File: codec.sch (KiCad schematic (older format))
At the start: 11 parts, among them U1 WM8778

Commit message: ksch: add stuff that isn't on soldered prototype yet
this hopefully completes the rev. A schematics
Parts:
- removed U1: WM8778, symbol WM8778
- removed U?: WM8778-units, symbol WM8778-units
- added C2: 0.1u, Capacitors_SMD:C_0805_HandSoldering, symbol C_Small
- added C3: 0.01u, Capacitors_SMD:C_0805_HandSoldering, symbol C_Small
- added C4: 1u, Capacitors_SMD:C_0805_HandSoldering, symbol C_Small
- added C5: 100p, Capacitors_SMD:C_0805_HandSoldering, symbol C_Small
- added C6, C7: 4.7nF, Capacitors_SMD:C_0805_HandSoldering, symbol C_Small
- added C8, C9: 10u, Capacitors_SMD:C_0805_HandSoldering, symbol C_Small
- added J1: electret mic, Socket_Strips:Socket_Strip_Straight_1x02_Pitch2.54mm, symbol CONN_01X02
- added J2: line in, Socket_Strips:Socket_Strip_Straight_1x03_Pitch2.54mm, symbol JACK_2P
- added J3: line/~mic, Connectors:GS2, symbol GS2
- added J5: JACK_3P, Socket_Strips:Socket_Strip_Straight_1x03_Pitch2.54mm, symbol JACK_3P
- added R10: 10k, Resistors_THT:R_Axial_DIN0207_L6.3mm_D2.5mm_P7.62mm_Horizontal, symbol R_Small
- added R11: 100k, Resistors_THT:R_Axial_DIN0207_L6.3mm_D2.5mm_P7.62mm_Horizontal, symbol R_Small
- added R12, R13: 680, Resistors_THT:R_Axial_DIN0207_L6.3mm_D2.5mm_P7.62mm_Horizontal, symbol R_Small
- added R5: 1k, Resistors_THT:R_Axial_DIN0207_L6.3mm_D2.5mm_P7.62mm_Horizontal, symbol R_Small
- added R6, R7: 2k, Resistors_THT:R_Axial_DIN0207_L6.3mm_D2.5mm_P7.62mm_Horizontal, symbol R_Small
- added R8, R9: 1M, Resistors_THT:R_Axial_DIN0207_L6.3mm_D2.5mm_P7.62mm_Horizontal, symbol R_Small
- added U2: MAX4466, TO_SOT_Packages_SMD:SOT-353_SC-70-5_Handsoldering, symbol MAX4466
- C401, C402: renamed from C?; footprint (none) -> Capacitors_THT:CP_Radial_D5.0mm_P2.00mm
- C403, C404: renamed from C?; footprint (none) -> Capacitors_THT:CP_Radial_D4.0mm_P2.00mm
- R401, R402, R403, R404: renamed from R?; footprint (none) -> Resistors_THT:R_Axial_DIN0207_L6.3mm_D2.5mm_P7.62mm_Horizontal
- U201: renamed from U?; footprint (none) -> footprints:SSOP-28_5.3x10.2mm_Pitch0.65mm_HandSolder
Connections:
- net labels removed: 3.3V, 5V, DGND
- wire segments 10 -> 46
- no-connect marks 28 -> 0
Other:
- note removed: "HIGH: I2S Mode\nLOW: 2pin Mode\nFLOAT: Hardware Mode"

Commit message: ksch: reannotate schematics to have a single style of part-naming
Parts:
- renumbered C2 to C34, C3 to C35, C4 to C36, C5 to C37, C6 to C38, C7 to C39, C8 to C40, C9 to C41, C401 to C42, C402 to C43, C403 to C44, C404 to C45, J1 to J5, J2 to J6, J3 to J7, J5 to J8, R7 to R10, R8 to R11, R9 to R12, R10 to R13, R11 to R14, R12 to R15, R13 to R16, R401 to R17, R402 to R18, R403 to R19, R404 to R20, R5 to R8, R6 to R9, U201 to U1, U2 to U7

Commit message: ksch: fix footprintproblem, change some labels
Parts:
- J8: value JACK_3P -> stereo_out
- U7: footprint TO_SOT_Packages_SMD:SOT-353_SC-70-5_Handsoldering -> footprints:SOT-353_SC-70-5_Handsoldering
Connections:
- net labels added: 5V, voutl, voutr
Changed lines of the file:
@@
 LIBS:ftdi
 LIBS:gennum
-LIBS:graphic
 LIBS:hc11
 LIBS:intel
@@
 LIBS:leds
 LIBS:linear
-LIBS:logo
 LIBS:maxim
 LIBS:mechanical
@@
 F 0 "U7" H 3550 2850 50  0000 L CNN
 F 1 "MAX4466" H 3550 2550 50  0000 L CNN
-F 2 "TO_SOT_Packages_SMD:SOT-353_SC-70-5_Handsoldering" H 3550 2550 50  0001 L CNN
+F 2 "footprints:SOT-353_SC-70-5_Handsoldering" H 3550 2550 50  0001 L CNN
 F 3 "" H 3700 2850 50  0001 C CNN
 	1    3550 2700
@@
 P 10050 3450
 F 0 "J8" H 9572 3433 50  0000 R CNN
-F 1 "JACK_3P" H 9572 3524 50  0000 R CNN
+F 1 "stereo_out" H 9572 3524 50  0000 R CNN
 F 2 "Socket_Strips:Socket_Strip_Straight_1x03_Pitch2.54mm" H 10050 3450 50  0001 C CNN
 F 3 "" H 10050 3450 50  0001 C CNN
@@
 Wire Wire Line
 	8650 3450 8650 3900
+Text Label 8850 3450 0    60   ~ 0
+voutl
+Text Label 8850 3100 0    60   ~ 0
+voutr
+Text GLabel 3450 2100 2    60   Input ~ 0
+5V
 $EndSCHEMATC

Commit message: k: fix pcb
power connector trouble
wrong footprint for caps
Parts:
- C44, C45: footprint Capacitors_THT:CP_Radial_D4.0mm_P2.00mm -> Capacitors_SMD:C_0805_HandSoldering
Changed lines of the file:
@@
 F 0 "C45" H 7960 4070 50  0000 L CNN
 F 1 "4.7nF" H 7960 3920 50  0000 L CNN
-F 2 "Capacitors_THT:CP_Radial_D4.0mm_P2.00mm" H 7950 4000 50  0001 C CNN
+F 2 "Capacitors_SMD:C_0805_HandSoldering" H 7950 4000 50  0001 C CNN
 F 3 "" H 7950 4000 50  0001 C CNN
 	1    7950 4000
@@
 F 0 "C44" H 7960 3270 50  0000 L CNN
 F 1 "4.7nF" H 7960 3120 50  0000 L CNN
-F 2 "Capacitors_THT:CP_Radial_D4.0mm_P2.00mm" H 7950 3200 50  0001 C CNN
+F 2 "Capacitors_SMD:C_0805_HandSoldering" H 7950 3200 50  0001 C CNN
 F 3 "" H 7950 3200 50  0001 C CNN
 	1    7950 3200

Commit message: ksch: change component values to include the unit except for resistors add more info to some devices
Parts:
- C34: value 0.1u -> 100nF
- C35: value 0.01u -> 10nF C0G/NP0
- C36: value 1u -> 1uF
- C37: value 100p -> 100pF
- C38, C39, C44, C45: value 4.7nF -> 4.7nF C0G/NP0
- C40, C41: value 10u -> 10uF C0G/NP0
- C42, C43: value 10uF -> 10uF C0G/NP0
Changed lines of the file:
@@
 Sheet 4 4
 Title "OpenLoop"
-Date "2017-09-25"
+Date "2017-10-02"
 Rev "A"
 Comp ""
@@
 P 7450 3900
 F 0 "C43" H 7475 4000 50  0000 L CNN
-F 1 "10uF" H 7475 3800 50  0000 L CNN
+F 1 "10uF C0G/NP0" H 7475 3800 50  0000 L CNN
 F 2 "Capacitors_THT:CP_Radial_D5.0mm_P2.00mm" H 7488 3750 50  0001 C CNN
 F 3 "" H 7450 3900 50  0001 C CNN
@@
 P 7950 4000
 F 0 "C45" H 7960 4070 50  0000 L CNN
-F 1 "4.7nF" H 7960 3920 50  0000 L CNN
+F 1 "4.7nF C0G/NP0" H 7960 3920 50  0000 L CNN
 F 2 "Capacitors_SMD:C_0805_HandSoldering" H 7950 4000 50  0001 C CNN
 F 3 "" H 7950 4000 50  0001 C CNN
@@
 P 7450 3100
 F 0 "C42" H 7475 3200 50  0000 L CNN
-F 1 "10uF" H 7475 3000 50  0000 L CNN
+F 1 "10uF C0G/NP0" H 7475 3000 50  0000 L CNN
 F 2 "Capacitors_THT:CP_Radial_D5.0mm_P2.00mm" H 7488 2950 50  0001 C CNN
 F 3 "" H 7450 3100 50  0001 C CNN
@@
 P 7950 3200
 F 0 "C44" H 7960 3270 50  0000 L CNN
-F 1 "4.7nF" H 7960 3120 50  0000 L CNN
+F 1 "4.7nF C0G/NP0" H 7960 3120 50  0000 L CNN
 F 2 "Capacitors_SMD:C_0805_HandSoldering" H 7950 3200 50  0001 C CNN
 F 3 "" H 7950 3200 50  0001 C CNN
@@
 P 3000 3100
 F 0 "C36" H 3010 3170 50  0000 L CNN
-F 1 "1u" H 3010 3020 50  0000 L CNN
+F 1 "1uF" H 3010 3020 50  0000 L CNN
 F 2 "Capacitors_SMD:C_0805_HandSoldering" H 3000 3100 50  0001 C CNN
 F 3 "" H 3000 3100 50  0001 C CNN
@@
 P 3450 3350
 F 0 "C37" H 3460 3420 50  0000 L CNN
-F 1 "100p" H 3460 3270 50  0000 L CNN
+F 1 "100pF" H 3460 3270 50  0000 L CNN
 F 2 "Capacitors_SMD:C_0805_HandSoldering" H 3450 3350 50  0001 C CNN
 F 3 "" H 3450 3350 50  0001 C CNN
@@
 P 2300 2600
 F 0 "C35" H 2310 2670 50  0000 L CNN
-F 1 "0.01u" H 2310 2520 50  0000 L CNN
+F 1 "10nF C0G/NP0" H 2310 2520 50  0000 L CNN
 F 2 "Capacitors_SMD:C_0805_HandSoldering" H 2300 2600 50  0001 C CNN
 F 3 "" H 2300 2600 50  0001 C CNN
@@
 P 1900 2750
 F 0 "C34" H 1910 2820 50  0000 L CNN
-F 1 "0.1u" H 1910 2670 50  0000 L CNN
+F 1 "100nF" H 1910 2670 50  0000 L CNN
 F 2 "Capacitors_SMD:C_0805_HandSoldering" H 1900 2750 50  0001 C CNN
 F 3 "" H 1900 2750 50  0001 C CNN
@@
 P 4450 3300
 F 0 "C38" H 4460 3370 50  0000 L CNN
-F 1 "4.7nF" H 4460 3220 50  0000 L CNN
+F 1 "4.7nF C0G/NP0" H 4460 3220 50  0000 L CNN
 F 2 "Capacitors_SMD:C_0805_HandSoldering" H 4450 3300 50  0001 C CNN
 F 3 "" H 4450 3300 50  0001 C CNN
@@
 P 4950 3350
 F 0 "C40" H 4960 3420 50  0000 L CNN
-F 1 "10u" H 4960 3270 50  0000 L CNN
+F 1 "10uF C0G/NP0" H 4960 3270 50  0000 L CNN
 F 2 "Capacitors_SMD:C_0805_HandSoldering" H 4950 3350 50  0001 C CNN
 F 3 "" H 4950 3350 50  0001 C CNN
@@
 P 4450 3750
 F 0 "C39" H 4460 3820 50  0000 L CNN
-F 1 "4.7nF" H 4460 3670 50  0000 L CNN
+F 1 "4.7nF C0G/NP0" H 4460 3670 50  0000 L CNN
 F 2 "Capacitors_SMD:C_0805_HandSoldering" H 4450 3750 50  0001 C CNN
 F 3 "" H 4450 3750 50  0001 C CNN
@@
 P 4950 3650
 F 0 "C41" H 4960 3720 50  0000 L CNN
-F 1 "10u" H 4960 3570 50  0000 L CNN
+F 1 "10uF C0G/NP0" H 4960 3570 50  0000 L CNN
 F 2 "Capacitors_SMD:C_0805_HandSoldering" H 4950 3650 50  0001 C CNN
 F 3 "" H 4950 3650 50  0001 C CNN

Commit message: migrate to kicad v5
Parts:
- C34, C35, C36, C37, C38, C39, C40, C41, C44, C45: symbol C_Small -> Device:C_Small
- C42, C43: symbol CP -> Device:CP
- J5: symbol CONN_01X02 -> Connector:Conn_01x02_Male
- J6: symbol JACK_2P -> Connector:AudioJack2_Ground_Switch
- J7: symbol GS2 -> Connector:TestPoint_2Pole
- J8: symbol JACK_3P -> openloop:JACK_3P
- R10, R11, R12, R13, R14, R15, R16, R17, R18, R19, R20, R8, R9: symbol R_Small -> Device:R_Small
- U1: symbol WM8778-units -> openloop:WM8778-units
- U7: symbol MAX4466 -> openloop:MAX4466
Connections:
- wire segments 46 -> 66

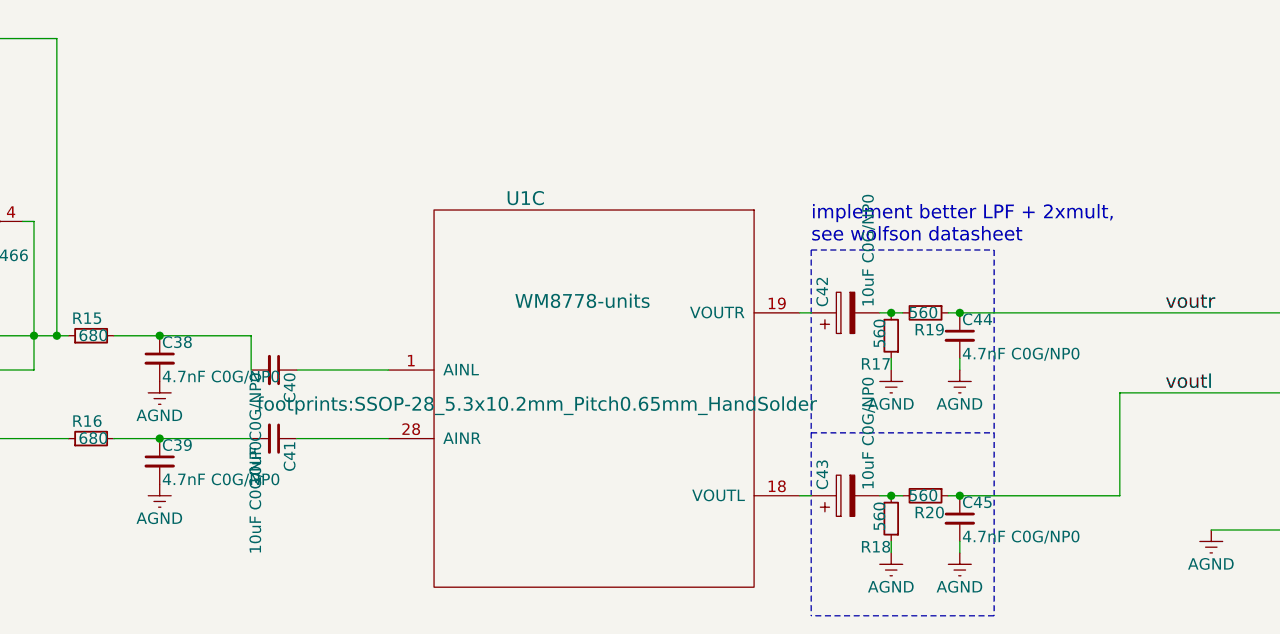
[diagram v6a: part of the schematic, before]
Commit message: ready for print
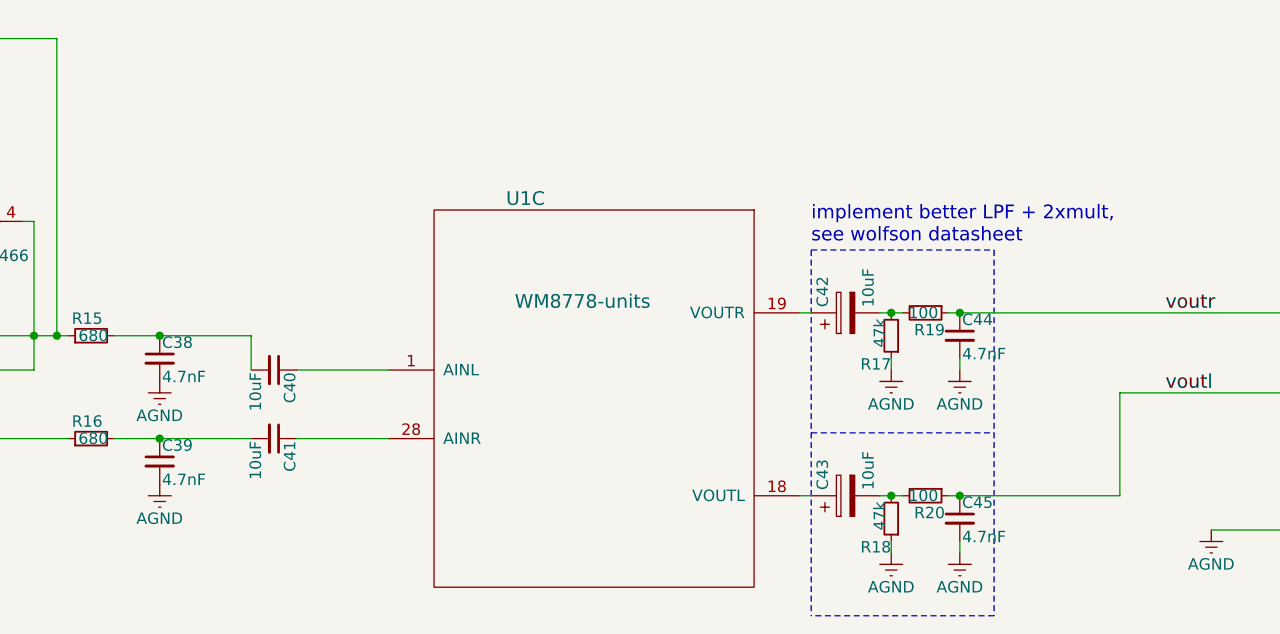
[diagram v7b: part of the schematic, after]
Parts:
- C38, C39, C44, C45: value 4.7nF C0G/NP0 -> 4.7nF
- C40, C41, C42, C43: value 10uF C0G/NP0 -> 10uF
- R17, R18: value 560 -> 47k
- R19, R20: value 560 -> 100
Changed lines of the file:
@@
 Sheet 4 4
 Title "OpenLoop"
-Date "2017-10-02"
+Date "2018-06-20"
 Rev "A"
 Comp ""
@@
 F 0 "U1" H 6050 4400 60  0000 C CNN
 F 1 "WM8778-units" H 6300 3950 60  0000 C CNN
-F 2 "footprints:SSOP-28_5.3x10.2mm_Pitch0.65mm_HandSolder" H 6100 3500 60  0000 C CNN
+F 2 "footprints:SSOP-28_5.3x10.2mm_Pitch0.65mm_HandSolder" H 6100 3500 60  0001 C CNN
 F 3 "" H 6100 3500 60  0000 C CNN
 	3    6350 3500
@@
 P 7800 3900
 F 0 "R20" V 7875 3850 50  0000 L CNN
-F 1 "560" V 7800 3825 50  0000 L CNN
+F 1 "100" V 7800 3825 50  0000 L CNN
 F 2 "Resistors_THT:R_Axial_DIN0207_L6.3mm_D2.5mm_P7.62mm_Horizontal" H 7800 3900 50  0001 C CNN
 F 3 "" H 7800 3900 50  0001 C CNN
@@
 P 7450 3900
 F 0 "C43" H 7475 4000 50  0000 L CNN
-F 1 "10uF C0G/NP0" H 7475 3800 50  0000 L CNN
+F 1 "10uF" H 7475 3800 50  0000 L CNN
 F 2 "Capacitors_THT:CP_Radial_D5.0mm_P2.00mm" H 7488 3750 50  0001 C CNN
 F 3 "" H 7450 3900 50  0001 C CNN
@@
 P 7950 4000
 F 0 "C45" H 7960 4070 50  0000 L CNN
-F 1 "4.7nF C0G/NP0" H 7960 3920 50  0000 L CNN
+F 1 "4.7nF" H 7960 3920 50  0000 L CNN
 F 2 "Capacitors_SMD:C_0805_HandSoldering" H 7950 4000 50  0001 C CNN
 F 3 "" H 7950 4000 50  0001 C CNN
@@
 P 7650 4000
 F 0 "R18" H 7650 4125 50  0000 L CNN
-F 1 "560" V 7700 3925 50  0000 L CNN
+F 1 "47k" V 7700 3925 50  0000 L CNN
 F 2 "Resistors_THT:R_Axial_DIN0207_L6.3mm_D2.5mm_P7.62mm_Horizontal" H 7650 4000 50  0001 C CNN
 F 3 "" H 7650 4000 50  0001 C CNN
@@
 P 7800 3100
 F 0 "R19" V 7875 3050 50  0000 L CNN
-F 1 "560" V 7800 3025 50  0000 L CNN
+F 1 "100" V 7800 3025 50  0000 L CNN
 F 2 "Resistors_THT:R_Axial_DIN0207_L6.3mm_D2.5mm_P7.62mm_Horizontal" H 7800 3100 50  0001 C CNN
 F 3 "" H 7800 3100 50  0001 C CNN
@@
 P 7450 3100
 F 0 "C42" H 7475 3200 50  0000 L CNN
-F 1 "10uF C0G/NP0" H 7475 3000 50  0000 L CNN
+F 1 "10uF" H 7475 3000 50  0000 L CNN
 F 2 "Capacitors_THT:CP_Radial_D5.0mm_P2.00mm" H 7488 2950 50  0001 C CNN
 F 3 "" H 7450 3100 50  0001 C CNN
@@
 P 7950 3200
 F 0 "C44" H 7960 3270 50  0000 L CNN
-F 1 "4.7nF C0G/NP0" H 7960 3120 50  0000 L CNN
+F 1 "4.7nF" H 7960 3120 50  0000 L CNN
 F 2 "Capacitors_SMD:C_0805_HandSoldering" H 7950 3200 50  0001 C CNN
 F 3 "" H 7950 3200 50  0001 C CNN
@@
 P 7650 3200
 F 0 "R17" H 7650 3325 50  0000 L CNN
-F 1 "560" V 7700 3125 50  0000 L CNN
+F 1 "47k" V 7700 3125 50  0000 L CNN
 F 2 "Resistors_THT:R_Axial_DIN0207_L6.3mm_D2.5mm_P7.62mm_Horizontal" H 7650 3200 50  0001 C CNN
 F 3 "" H 7650 3200 50  0001 C CNN
@@
 P 4450 3300
 F 0 "C38" H 4460 3370 50  0000 L CNN
-F 1 "4.7nF C0G/NP0" H 4460 3220 50  0000 L CNN
+F 1 "4.7nF" H 4460 3220 50  0000 L CNN
 F 2 "Capacitors_SMD:C_0805_HandSoldering" H 4450 3300 50  0001 C CNN
 F 3 "" H 4450 3300 50  0001 C CNN
@@
 P 4950 3350
 F 0 "C40" H 4960 3420 50  0000 L CNN
-F 1 "10uF C0G/NP0" H 4960 3270 50  0000 L CNN
+F 1 "10uF" H 4960 3270 50  0000 L CNN
 F 2 "Capacitors_SMD:C_0805_HandSoldering" H 4950 3350 50  0001 C CNN
 F 3 "" H 4950 3350 50  0001 C CNN
@@
 P 4450 3750
 F 0 "C39" H 4460 3820 50  0000 L CNN
-F 1 "4.7nF C0G/NP0" H 4460 3670 50  0000 L CNN
+F 1 "4.7nF" H 4460 3670 50  0000 L CNN
 F 2 "Capacitors_SMD:C_0805_HandSoldering" H 4450 3750 50  0001 C CNN
 F 3 "" H 4450 3750 50  0001 C CNN
@@
 P 4950 3650
 F 0 "C41" H 4960 3720 50  0000 L CNN
-F 1 "10uF C0G/NP0" H 4960 3570 50  0000 L CNN
+F 1 "10uF" H 4960 3570 50  0000 L CNN
 F 2 "Capacitors_SMD:C_0805_HandSoldering" H 4950 3650 50  0001 C CNN
 F 3 "" H 4950 3650 50  0001 C CNN

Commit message: update codec schematic: mic power
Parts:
- removed C35: 10nF C0G/NP0, Capacitors_SMD:C_0805_HandSoldering, symbol Device:C_Small
- removed C44, C45: 4.7nF, Capacitors_SMD:C_0805_HandSoldering, symbol Device:C_Small
- removed J7: line/~mic, Connectors:GS2, symbol Connector:TestPoint_2Pole
- J5: symbol Connector:Conn_01x02_Male -> Connector:Conn_01x03_Male
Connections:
- wire segments 66 -> 55
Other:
- note removed: "implement better LPF + 2xmult, \nsee wolfson datasheet"
- moved on the sheet: C34, C36, C37, C38, C39, C40, C41, J6, R10, R11, R12, R13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
